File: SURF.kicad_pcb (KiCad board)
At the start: 2 copper layers, 33 x 30.5 mm, 31 parts, among them IC1 TPS7A0212PDBVR, IC2 TPS7A0228PDBVR, J1 Conn_01x10_Pin RIGHT, J2 Conn_01x10_Pin LEFT, J3 Conn_01x04, Q3 Q_Dual_PMOS_S1G1D2S2G2D1, U1 ESP32-S2-MINI-2

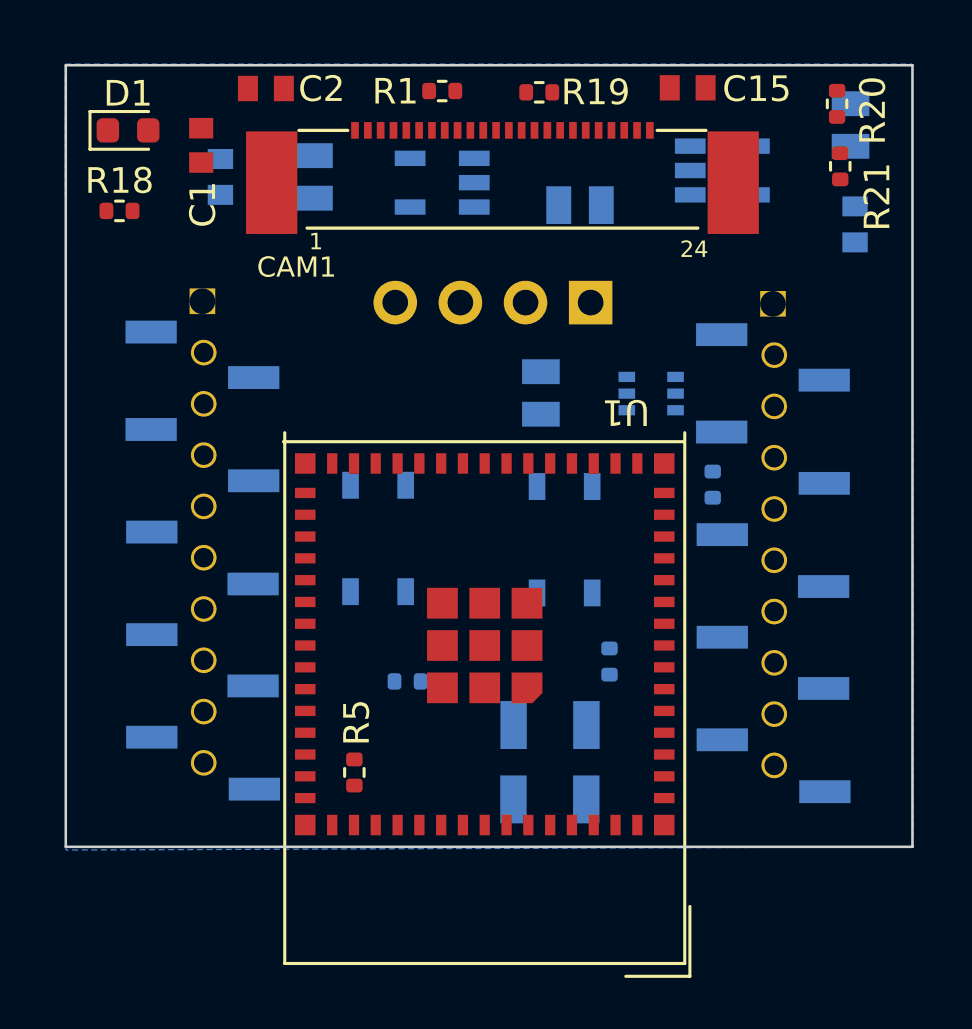
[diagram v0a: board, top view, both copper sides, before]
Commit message: new update
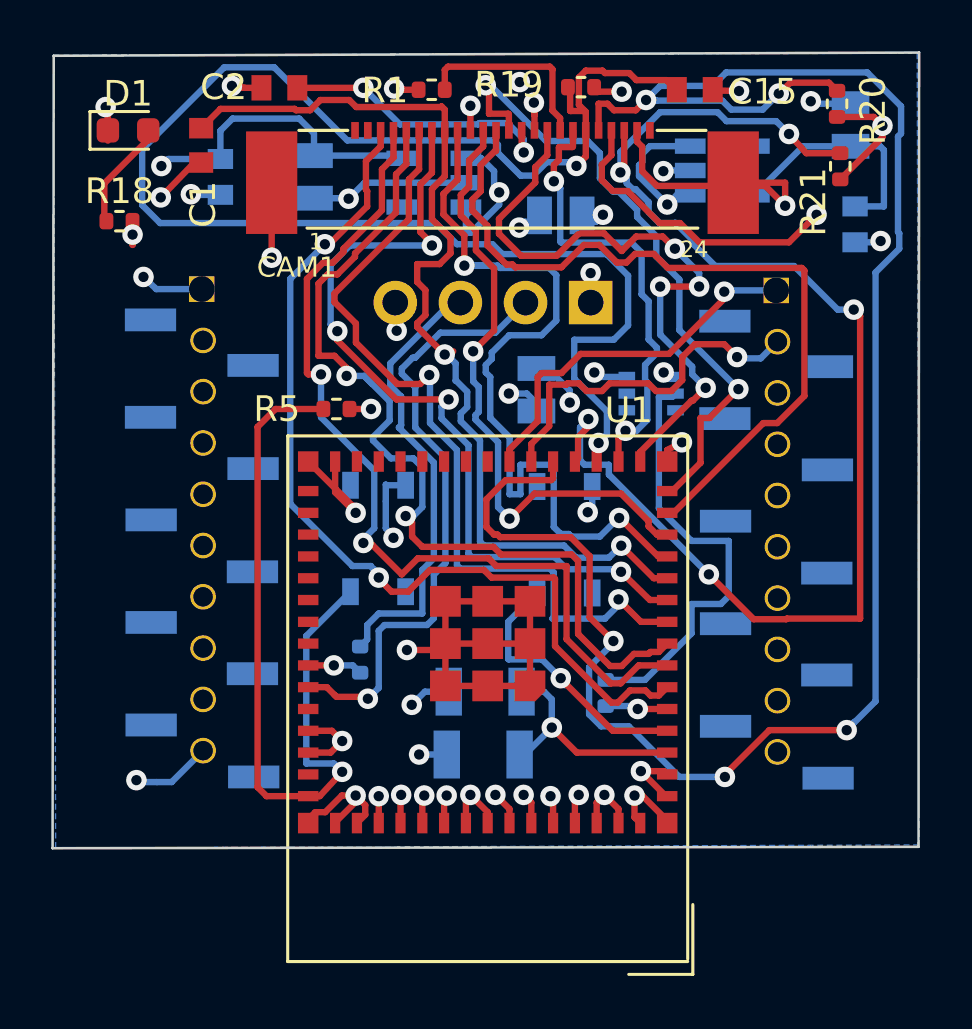
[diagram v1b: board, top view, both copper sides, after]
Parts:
- removed R23: 10K, Resistor_SMD:R_0402_1005Metric
- moved R5 14.2 mm to (170.6, 84.5), turned to 0 degrees
- moved C4 3.13 mm to (176.3, 98.0)
- moved C5 2.84 mm to (176.4, 95.5)
- moved R4 2.04 mm to (171.5, 94.3), turned to -90 degrees
- moved R19 1.64 mm to (180.1, 72.0)
- moved R24 1.23 mm to (181.1, 95.6)
- moved C18 0.85 mm to (179.3, 77.0)
- moved J1 0.54 mm to (184.0, 72.4)
- moved C2 0.53 mm to (168.3, 72.0), turned to 180 degrees
- moved J2 0.48 mm to (161.6, 72.3)
- moved R1 0.41 mm to (174.3, 72.1)
- moved R18 0.40 mm to (162.1, 77.2)
- moved IC1 0.32 mm to (174.4, 75.7)
- moved C15 0.29 mm to (184.6, 72.1)
- moved C17 0.22 mm to (178.4, 83.8)
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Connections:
- CAM1 pad P$25: (no net) -> GND
- CAM1 pad P$26: (no net) -> GND
- CAM1 pad P1: (no net) -> unnconnected
- CAM1 pad P10: (no net) -> GND
- CAM1 pad P11: (no net) -> /GPIO9
- CAM1 pad P12: (no net) -> /GPIO10
- CAM1 pad P13: (no net) -> /GPIO11
- CAM1 pad P14: (no net) -> /CAM_VCC
- CAM1 pad P15: (no net) -> +1V2
- CAM1 pad P16: (no net) -> /GPIO12
- CAM1 pad P17: (no net) -> /PWDN
- CAM1 pad P18: (no net) -> /GPIO13
- CAM1 pad P19: (no net) -> /GPIO14
- CAM1 pad P2: (no net) -> unnconnected
- CAM1 pad P20: (no net) -> /TWI_SCK
- CAM1 pad P21: (no net) -> +2V8
- CAM1 pad P22: (no net) -> /TWI_SDA
- CAM1 pad P23: (no net) -> GND
- CAM1 pad P24: (no net) -> unnconnected
- CAM1 pad P3: (no net) -> /GPIO2
- CAM1 pad P4: (no net) -> /GPIO3
- CAM1 pad P5: (no net) -> /GPIO4
- CAM1 pad P6: (no net) -> /GPIO5
- CAM1 pad P7: (no net) -> /GPIO6
- CAM1 pad P8: (no net) -> /GPIO7
- CAM1 pad P9: (no net) -> /GPIO8
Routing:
- net GND: track 0.00 -> 102.3 mm, vias 0 -> 38
- net /TWI_SCK: track 0.00 -> 76.6 mm, vias 0 -> 5
- net /GPIO14: track 0.00 -> 61.8 mm, vias 0 -> 2
- net /TWI_SDA: track 0.00 -> 54.0 mm, vias 0 -> 5
- net /GPIO7: track 0.00 -> 38.8 mm, vias 0 -> 2
- net /GPIO2: track 0.00 -> 36.8 mm, vias 0 -> 2
- net /GPIO3: track 0.00 -> 36.5 mm, vias 0 -> 2
- net /GPIO4: track 0.00 -> 36.0 mm, vias 0 -> 2
- net /GPIO6: track 0.00 -> 32.8 mm, vias 0 -> 4
- net /GPIO5: track 0.00 -> 32.8 mm, vias 0 -> 2
- net /GPIO8: track 0.00 -> 32.3 mm, vias 0 -> 2
- net /GPIO10: track 0.00 -> 31.1 mm
- net /EN: track 0.00 -> 29.9 mm, vias 0 -> 1
- net /GPIO11: track 0.00 -> 25.1 mm, vias 0 -> 2
- net /GPIO12: track 0.00 -> 25.0 mm, vias 0 -> 4
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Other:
- board size 33 x 30.5 mm -> 33.8 x 31 mm

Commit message: new update
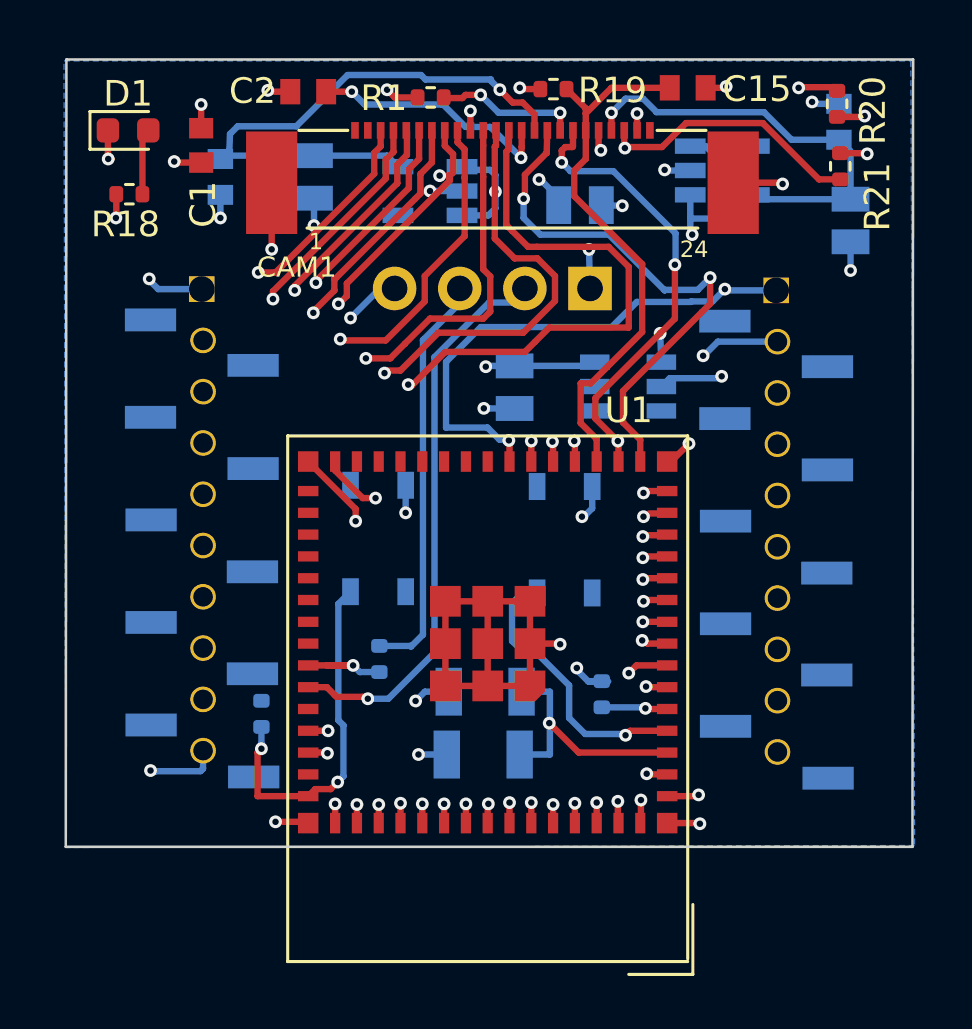
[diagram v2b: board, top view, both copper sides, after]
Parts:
- Q3: value Q_Dual_PMOS_S1G1D2S2G2D1 -> DMP3098LDM-7; footprint Package_TO_SOT_SMD:SOT-363_SC-70-6 -> DMP3098LDM-7:SOT95P285X140-6N
- R5: moved to B.Cu
- moved R5 12.2 mm to (167.7, 96.4), turned to 90 degrees
- moved C20 4.05 mm to (190.2, 73.3), turned to 90 degrees
- moved C19 3.72 mm to (190.6, 77.2), turned to -90 degrees
- moved C2 1.13 mm to (169.5, 72.2)
- moved R18 1.12 mm to (162.5, 76.2), turned to 180 degrees
- moved R19 1.08 mm to (179.0, 72.0), turned to 180 degrees
- moved Q3 0.94 mm to (181.9, 83.7)
- moved C17 0.86 mm to (177.5, 83.7)
- moved C18 0.85 mm to (180.1, 76.6)
- moved R4 0.75 mm to (172.2, 94.3)
- moved J3 0.55 mm to (180.5, 79.8)
- moved IC1 0.36 mm to (174.2, 76.0)
- moved R1 0.30 mm to (174.2, 72.4)
- moved C15 0.29 mm to (184.3, 72.0)
- moved R24 0.16 mm to (180.9, 95.7)
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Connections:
- C17 pad 1: VCC -> +3V0
- J2 pad 1: VCC -> +3V0
- Q3 pad 6: VCC -> +3V0
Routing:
- net /TWI_SCK: track 76.6 -> 28.1 mm, vias 5 -> 3
- net /GPIO14: track 61.8 -> 21.3 mm, vias 2 -> 0
- net /CAM_VCC: track 23.7 -> 55.0 mm, vias 7 -> 6
- net /TWI_SDA: track 54.0 -> 24.9 mm, vias 5 -> 2
- net GND: track 102.3 -> 74.7 mm, vias 38 -> 48
- net /GPIO11: track 25.1 -> 43.5 mm
- net /EN: track 29.9 -> 14.1 mm, vias 1 -> 2
- net /GPIO9: track 24.4 -> 36.8 mm
- net /GPIO7: track 38.8 -> 48.6 mm, vias 2 -> 4
- net /GPIO10: track 31.1 -> 40.4 mm, vias 0 -> 2
- net +1V2: track 14.7 -> 22.5 mm, vias 2 -> 1
- net VCC: track 6.23 -> 0.00 mm, vias 3 -> 0
- net /GPIO18: track 14.8 -> 20.1 mm, vias 1 -> 2
- net +2V8: track 21.1 -> 16.8 mm
- net +3V0: track 18.5 -> 22.7 mm, vias 6 -> 8
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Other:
- board size 33.8 x 31 mm -> 33 x 30.7 mm
- copper layers 2 -> 4
